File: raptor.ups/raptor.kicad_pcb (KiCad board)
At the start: 2 copper layers, 10 parts, among them P1 CONN_220V, P2 CONN_RPI, P3 CONN_HUB, P4 Power

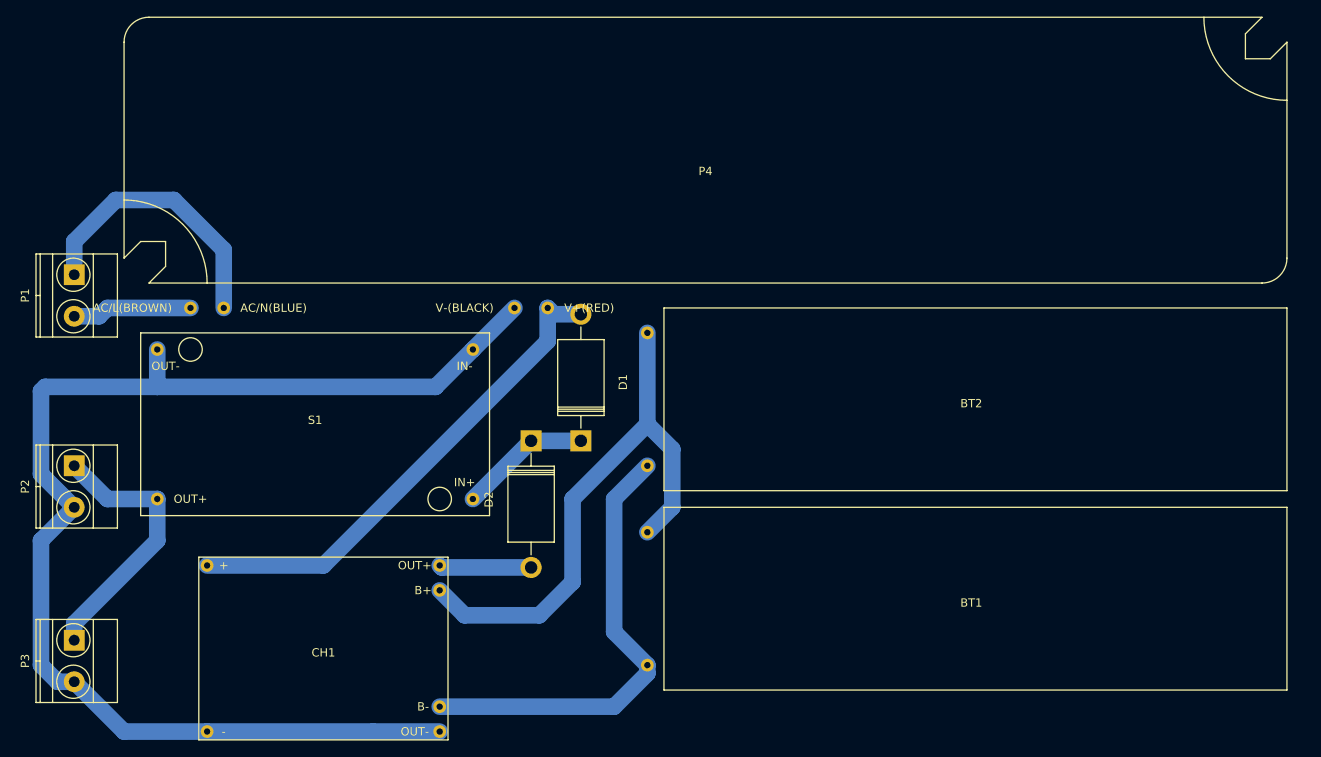
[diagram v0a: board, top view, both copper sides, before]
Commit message: Jeszcze poprawki płytki PCB UPS-a.
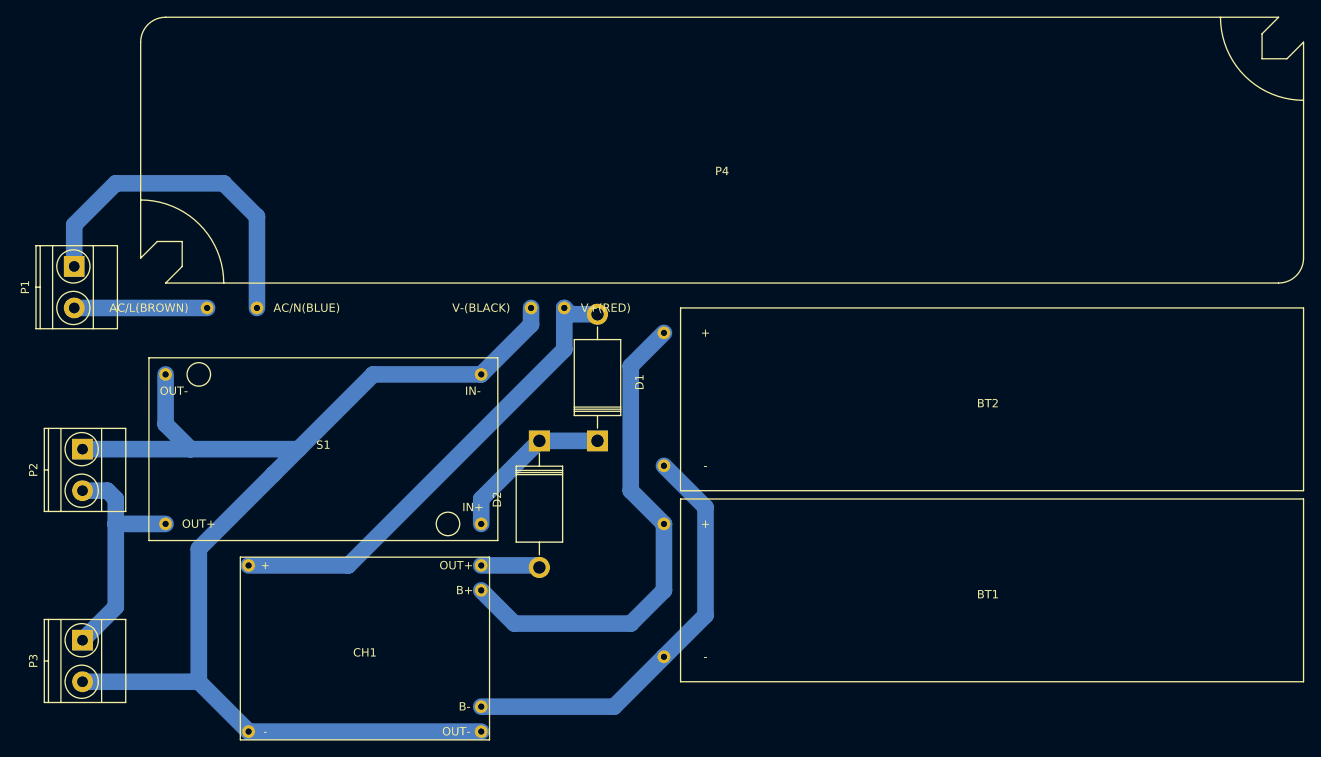
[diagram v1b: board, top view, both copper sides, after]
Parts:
- moved CH1 5.00 mm to (117.0, 118.0)
- moved S1 3.16 mm to (112.0, 94.0)
- moved BT1 2.24 mm to (192.0, 111.0)
- moved P2 2.24 mm to (83.0, 94.0)
- moved BT2 2.00 mm to (192.0, 88.0)
- moved D1 2.00 mm to (145.0, 93.0)
- moved P4 2.00 mm to (160.0, 58.0)
- moved D2 1.00 mm to (138.0, 93.0)
- moved P1 1.00 mm to (82.0, 72.0)
- moved P3 1.00 mm to (83.0, 117.0)
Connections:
- P2 pad 1: Net-(P2-Pad1) -> GND
- P2 pad 2: GND -> Net-(P2-Pad2)
- P3 pad 1: Net-(P2-Pad1) -> Net-(P2-Pad2)
- S1 pad 3: Net-(P2-Pad1) -> Net-(P2-Pad2)
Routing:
- net Net-(P2-Pad1): track 32.8 -> 0.00 mm
- net Net-(P2-Pad2): track 0.00 -> 29.1 mm
- net Net-(BT1-Pad1): track 68.1 -> 59.6 mm
- net Net-(P1-Pad1): track 33.6 -> 41.7 mm
- net Net-(D1-Pad1): track 15.9 -> 19.9 mm
- net Net-(CH1-Pad3): track 11.1 -> 7.44 mm
- net Net-(BT1-Pad2): track 55.0 -> 51.6 mm
- net GND: track 153.3 -> 155.9 mm
- net VCC: track 60.5 -> 58.1 mm
- net Net-(P1-Pad2): track 14.4 -> 16.0 mm
